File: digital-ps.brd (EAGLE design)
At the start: 82.5 x 54.6 mm, 106 parts, among them CON1 SWD_CON, IC1 7805, IC2 3.3V, IC3 STM32F334K8, IC4 OPA, IC5 MCP14700, Q1 EPC2052, Q2 EPC2052, T1 COMMON_FILTER-SMALL, X1 12MHz

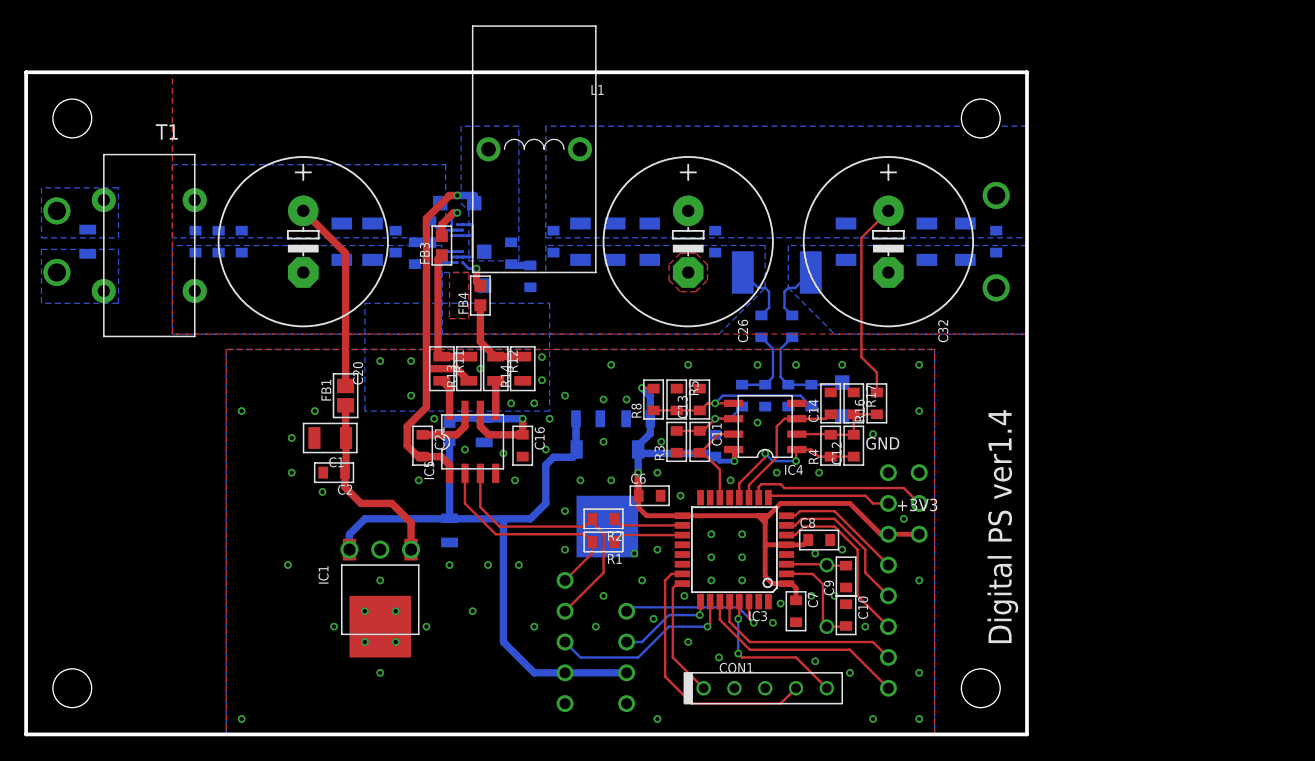
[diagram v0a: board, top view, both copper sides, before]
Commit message: Si
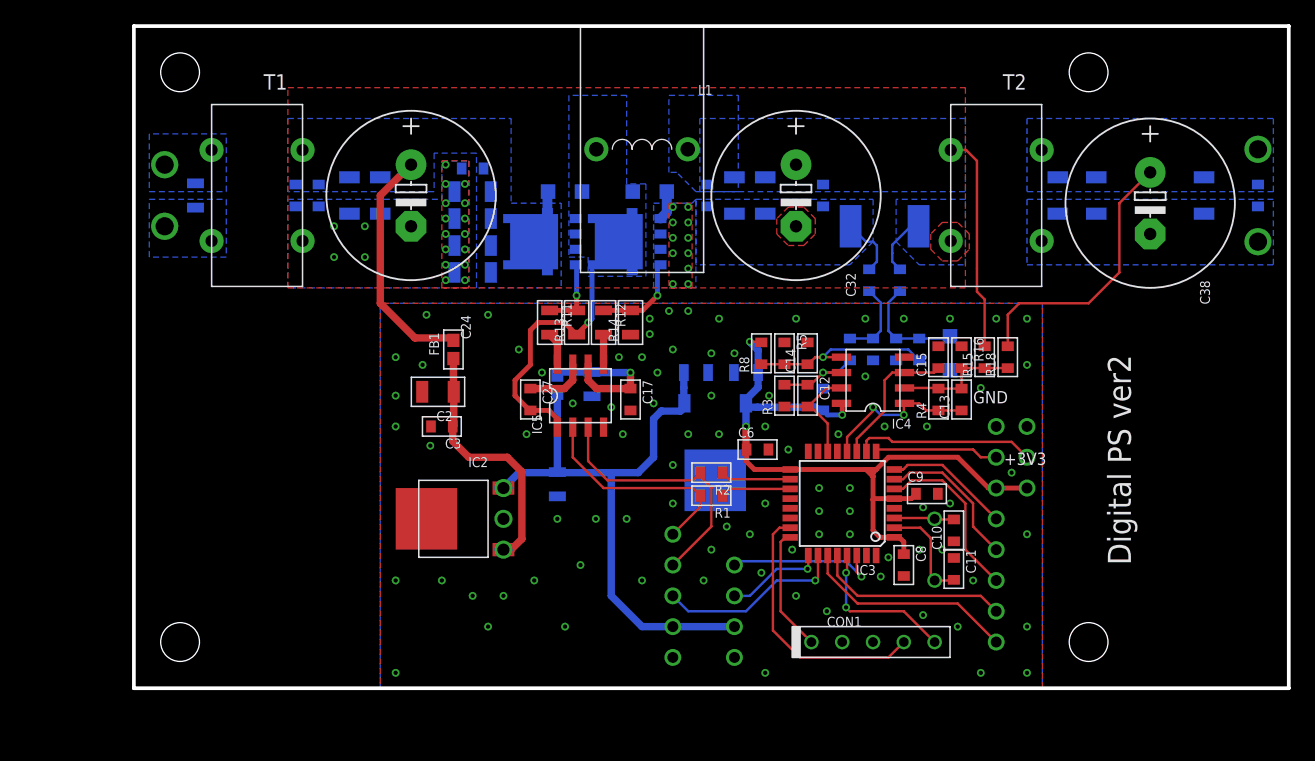
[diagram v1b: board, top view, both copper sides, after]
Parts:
- removed FB3, FB4: FB, my_rcl:1608-FB
- removed R19: 2, my_rcl:1608-2
- added T2: COMMON_FILTER-SMALL, my_rcl:COMMON_FILTER__SMALL
- C1: value 10u -> 1u; device my_rcl:3216 -> my_rcl:2012-2
- C11: value 1000p -> 10p
- C15: value 10u -> 1000p; device my_rcl:2012 -> my_rcl:1608
- C16, C7: value 0.1u -> 10u; device my_rcl:1608 -> my_rcl:2012
- C17: value 1000p -> 0.1u
- C18: value 1000p -> 1u; device my_rcl:1608 -> my_rcl:1608-2
- C19: value 0.1u -> 1u; device my_rcl:1608 -> my_rcl:1608-2
- C2: value 0.1u -> 10u; device my_rcl:1608 -> my_rcl:3216
- C20: value 1000u -> 1000p; device my_rcl:E5-13 -> my_rcl:1608
- C21: value 0.1u -> 1000p
- C22, C33, C34: value 10u -> 1u; device my_rcl:3225-2 -> my_rcl:1608-2
- C23: value 10u -> 0.1u; device my_rcl:3225-2 -> my_rcl:1608
- C24: value 1u -> 1000u; device my_rcl:1608-2 -> my_rcl:E5-13
- C25: value 1n -> 10u; device my_rcl:1608-2 -> my_rcl:3225-2
- C26: value DNP -> 10u; device my_rcl:E5-13 -> my_rcl:3225-2
- C27: value 1u -> 0.1u; device my_rcl:1608-2 -> my_rcl:1608
- C3: value 10u -> 0.1u; device my_rcl:2012 -> my_rcl:1608
- C30: value 10u -> 1u
- C31: value 10u -> 0.1u
- C35, C36, C37, C39, C40: value 1u -> 10u; device my_rcl:1608-2 -> my_rcl:3225-2
- C38: value 0.1u -> 470u; device my_rcl:1608-2 -> my_rcl:E5-13
- C41: device my_rcl:2012-2 -> my_rcl:1608-2
- C9: value 10p -> 0.1u
- FB1: value FB-2012 -> FB-1608FB; device my_rcl:2012-J -> my_rcl:1608-FB
- IC1: value 7805 -> 3.3V; device my_ic:TO220-SOP-DUAL -> my_ic:P-HSIP3_2.30A
- IC2: value 3.3V -> 7805; device my_ic:P-HSIP3_2.30A -> my_ic:TO220-SOP-DUAL
- Q1, Q2: device my_ic:EPC2052 -> my_ic:DFN5_5X6
- R10, R9: value 100 -> 39
- R15: value 10 -> 10k; device my_rcl:1608-2 -> my_rcl:1608
- R16: value 10k -> 1k
- R17: value 1k -> 10m; device my_rcl:1608 -> my_rcl:6432
- R18: value 10m -> DNP; device my_rcl:6432 -> my_rcl:1608
- moved C41 96.6 mm to (92.7, 40.6)
- moved C37 71.2 mm to (76.2, 40.6)
- moved C38 60.8 mm to (83.8, 40.0), flipped to the top
- moved C20 47.8 mm to (61.0, 27.9), flipped to the bottom, turned to 90 degrees
- moved C35 45.2 mm to (52.1, 40.6)
- moved C18 43.9 mm to (13.3, 40.6)
- moved C31 40.8 mm to (27.9, 41.0), turned to 0 degrees
- moved C36 40.8 mm to (49.5, 40.6)
- moved R15 40.0 mm to (70.2, 27.3), flipped to the top
- moved C21 39.9 mm to (62.9, 27.9), flipped to the bottom
- moved C23 39.4 mm to (56.8, 23.8), turned to 90 degrees
- moved C15 37.9 mm to (66.4, 27.3), flipped to the top, turned to 90 degrees
- moved C39 31.7 mm to (79.4, 40.6)
- moved C19 30.4 mm to (27.9, 42.9), turned to 0 degrees
- moved IC1 30.1 mm to (47.9, 23.5), flipped to the bottom
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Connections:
- removed net N$10: FB4.2, Q2.1
- removed net N$28: C25.1, R15.1
- removed net N$34: C38.1, R19.1
- removed net N$9: FB3.2, Q1.1
- new net ISENSE: R10.2, R17.2, T2.1
- new net OUT: C32.+, C33.1, C34.1, C35.1, C36.1, L1.2, R15.2, T2.4
- net +3V3: now also C23.1, C9.1, IC1.3; no longer C19.1, C7.1, IC2.3
- net +5V: now also C7.1, IC1.1, IC2.3, IC2.6; no longer C3.1, IC1.3, IC1.6, IC2.1
- net +5VP: now also C17.1; no longer C15.1
- net GND: now also C11.1, C17.2, C20.1, C21.2, C24.-, C26.2, C31.2, C32.-, C33.2, C34.2, C9.2, IC2.5, Q2.1, R16.1; no longer C1.2, C13.2, C17.1, C20.-, C24.2, C26.-, C27.2, C37.2, C38.2, C39.2, C9.1, IC1.5, Q2.7, Q2.8, Q2.9, R18.1
- net IN+: now also C1.1; no longer C41.1
- net IN-: now also C1.2; no longer C41.2
- net N$11: now also C21.1; no longer C18.1
- net N$24: now also C11.2; no longer C10.2
- net N$25: now also C10.2; no longer C9.2
- net N$29: now also C12.1; no longer C11.1
- net N$3: now also C12.2; no longer C11.2
- net N$30: now also C13.1; no longer C12.1
- net N$31: now also C15.1; no longer C14.1
- net N$32: now also Q1.4; no longer FB3.1
- net N$33: now also Q2.4; no longer FB4.1
- net N$4: now also C3.1, IC2.1, IC2.4; no longer C1.1, IC1.1, IC1.4
- net N$5: now also C14.1; no longer C13.1
- net N$7: now also C27.1; no longer C21.1
- net N$8: now also C20.2; no longer C17.2
- net OUT+: now also C37.1, C38.+, C41.1, R18.2, T2.3; no longer C26.+, C27.1, C28.1, C29.1, C30.1, C31.1, C32.+, C33.1, C34.1, L1.2, R16.2
- net OUT-: now also C37.2, C38.-, C39.2, C41.2, T2.2; no longer C31.2, C32.-, C33.2, C34.2, R10.2, R18.2
- net SW: now also C27.2, Q1.1, Q2.5_6, Q2.5_6_1, Q2.5_6_2, Q2.5_6_3, Q2.5_6_4; no longer C21.2, Q1.7, Q1.8, Q1.9, Q2.4, Q2.5, Q2.6, R15.2
- net VFB: now also C13.2, R15.1, R16.2, R18.1; no longer C12.2, R16.1, R17.2
- net VP: now also C18.1, C19.1, C24.+, C25.1, C26.1, C28.1, C29.1, C30.1, C31.1, Q1.5_6, Q1.5_6_1, Q1.5_6_2, Q1.5_6_3, Q1.5_6_4; no longer C20.+, C23.1, C24.1, C35.1, C36.1, C37.1, Q1.4, Q1.5, Q1.6, R19.2
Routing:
- net SW: track 40.9 -> 21.7 mm
- net OUT: track 0.00 -> 18.1 mm
- net OUT+: track 16.4 -> 22.6 mm
- net N$4: track 15.7 -> 21.0 mm
- net +5V: track 55.4 -> 50.3 mm
- net ISENSE: track 0.00 -> 5.08 mm
- net OUT-: track 5.04 -> 0.00 mm
- net N$32: track 10.8 -> 6.01 mm, vias 0 -> 1
- net N$9: track 3.78 -> 0.00 mm, vias 1 -> 0
- net N$10: track 2.90 -> 0.00 mm, vias 1 -> 0
- net VP: track 18.9 -> 21.4 mm
- net GND: track 9.57 -> 7.48 mm, vias 88 -> 118
- net VFB: track 8.32 -> 10.2 mm
- net N$28: track 1.63 -> 0.00 mm
- net N$34: track 1.29 -> 0.00 mm
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- added copper zone on layer 15, net GND
- added copper zone on layer 2, net GND
- added copper zone on layer 16, net ISENSE
- added copper zone on layer 16, net OUT
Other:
- board size 82.5 x 54.6 mm -> 95.2 x 54.6 mm
- board text added: "Digital PS ver2"
- board text removed: "Digital PS ver1.4"
